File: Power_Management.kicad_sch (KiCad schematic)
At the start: 16 parts, among them J2 I2S_OR_LJ_OUT, Q1 MOSFET_SI2333DDS-T1-BE3, U4 SN74LVC1G07DBVR

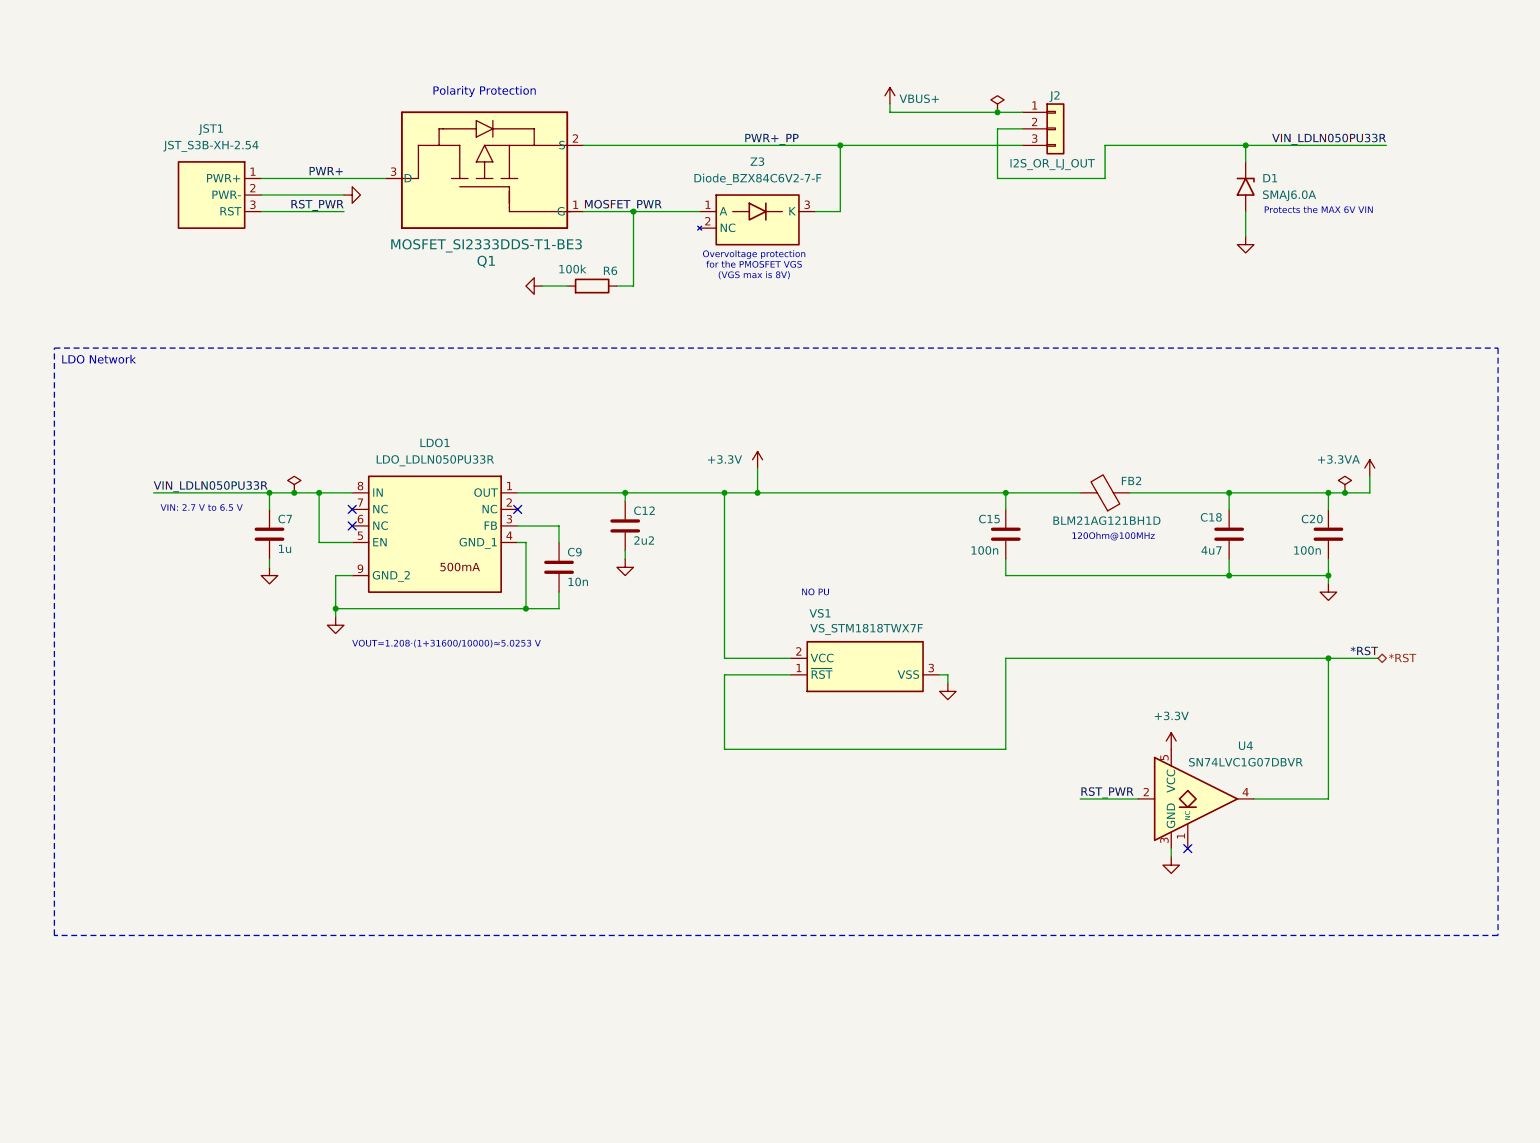
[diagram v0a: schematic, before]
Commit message: JLCPCB Check
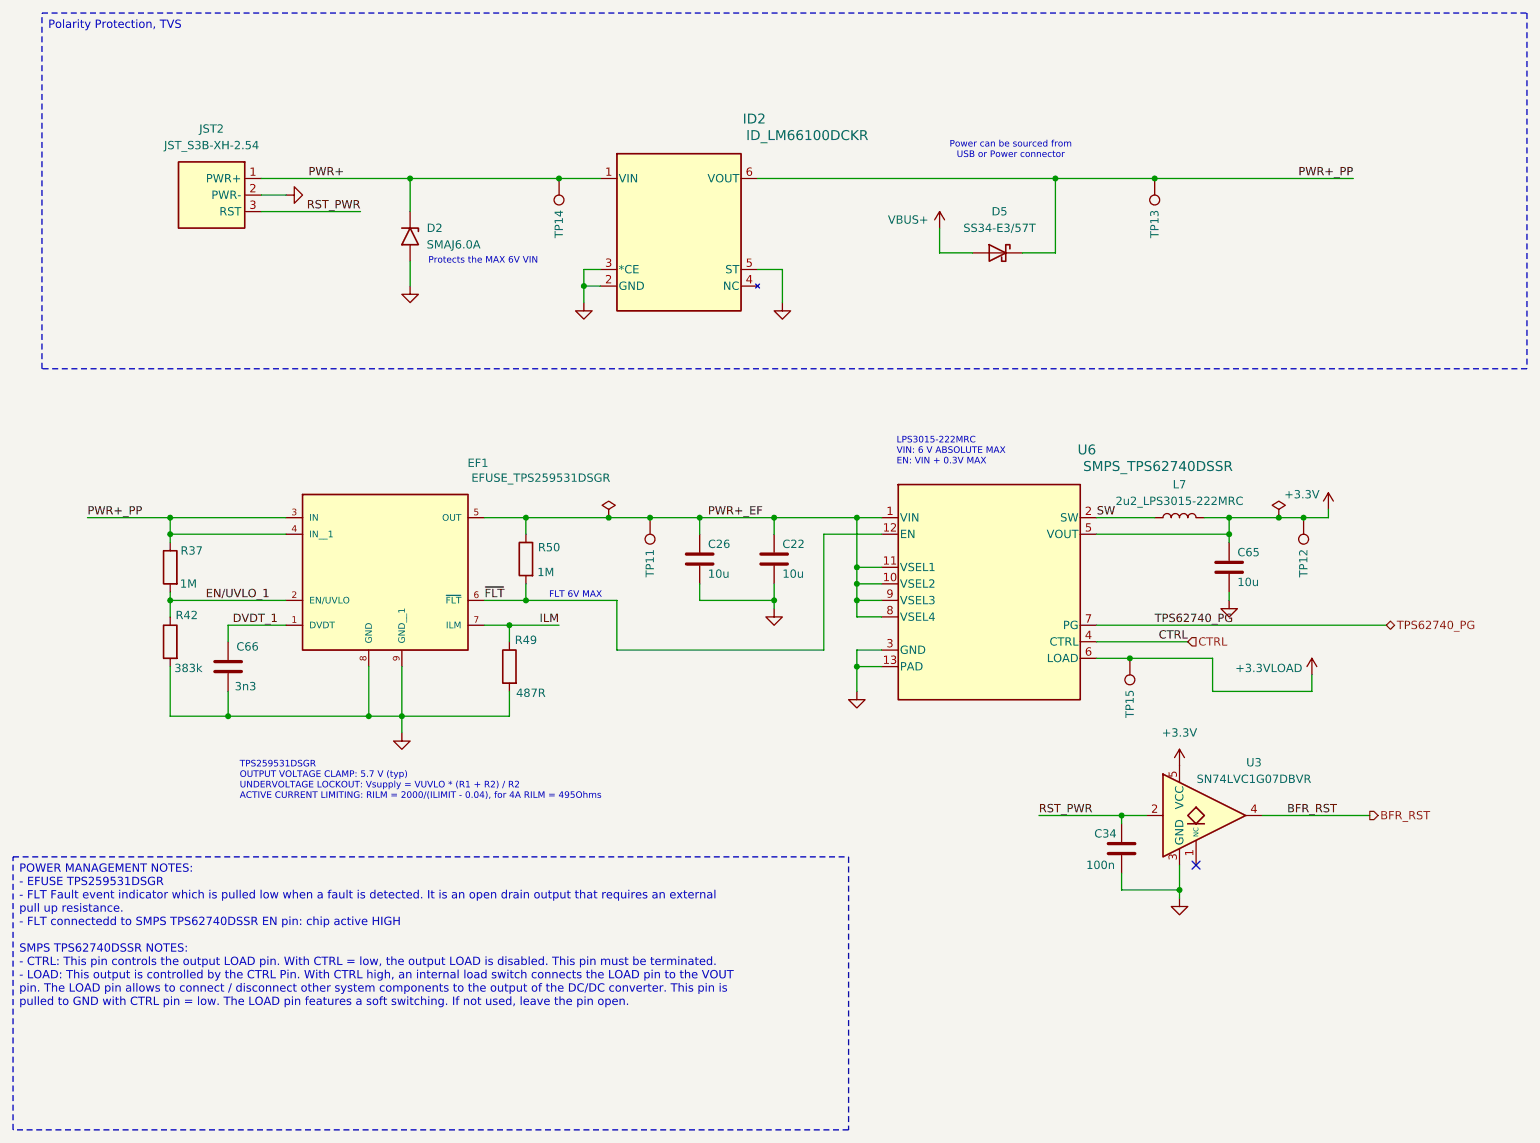
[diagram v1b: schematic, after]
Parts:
- removed C12: 2u2, Capacitor_SMD:C_0805_2012Metric, symbol Device:C
- removed C15, C20: 100n, Capacitor_SMD:C_0805_2012Metric, symbol Device:C
- removed C18: 4u7, Capacitor_SMD:C_0805_2012Metric, symbol Device:C
- removed C7: 1u, Capacitor_SMD:C_0805_2012Metric, symbol Device:C
- removed C9: 10n, Capacitor_SMD:C_0805_2012Metric, symbol Device:C
- removed D1: SMAJ6.0A, Personal_Project:DO-214AC-2, symbol Personal_Projects:DIODE_SMAJ6.0A
- removed FB2: BLM21AG121BH1D, Capacitor_SMD:C_0805_2012Metric, symbol Device:FerriteBead
- removed J2: I2S_OR_LJ_OUT, Connector_PinHeader_2.54mm:PinHeader_1x03_P2.54mm_Vertical, symbol Connector_Generic:Conn_01x03
- removed JST1: JST_S3B-XH-2.54, Personal_Project:JST_S3B-XH-SHDRRA3W64P0X250_1X3_990X1150X610P, symbol Personal_Projects:JST_S3B-XH-A-1_LF_SN
- removed LDO1: LDO_LDLN050PU33R, Package_DFN_QFN:DFN-8-1EP_3x3mm_P0.65mm_EP1.7x2.05mm, symbol Personal_Projects:LDO_LDLN050PUR
- removed Q1: MOSFET_SI2333DDS-T1-BE3, Personal_Project:MOSFET_ SI2333DDS_SOT_DS-T1-BE3_VIS, symbol Personal_Projects:MOSFET_SI2333DDS-T1-BE3
- removed R6: 100k, Resistor_SMD:R_0805_2012Metric, symbol Device:R
- removed U4: SN74LVC1G07DBVR, Package_TO_SOT_SMD:SOT-23-5, symbol 74xGxx:74LVC1G07
- removed VS1: VS_STM1818TWX7F, Personal_Project:SOT-23-3_SOT103P237X112-3N, symbol Personal_Projects:VS_STM1813LWX7F
- removed Z3: Diode_BZX84C6V2-7-F, Personal_Project:Diode_BZX84C6V2_SOT96P240X110-3N, symbol Personal_Projects:Diode_BZX84C6V2-7-F
- added C22, C26, C65: 10u, Capacitor_SMD:C_0603_1608Metric, symbol Device:C
- added C34: 100n, Capacitor_SMD:C_0805_2012Metric, symbol Device:C
- added C66: 3n3, Capacitor_SMD:C_0603_1608Metric, symbol Device:C
- added D2: SMAJ6.0A, Personal_Project:DO-214AC-2, symbol Personal_Projects:DIODE_SMAJ6.0A
- added D5: SS34-E3/57T, Diode_SMD:D_SMA, symbol Diode:SS34
- added EF1: EFUSE_TPS259531DSGR, Personal_Projects:EF_TPS259531DSGR, symbol Personal_Components:EFUSE_TPS259531DSGR
- added ID2: ID_LM66100DCKR, Personal_Projects:ID_LM66100DCKR, symbol Personal_Components:ID_LM66100DCKR
- added JST2: JST_S3B-XH-2.54, Personal_Project:JST_S3B-XH-SHDRRA3W64P0X250_1X3_990X1150X610P, symbol Personal_Projects:JST_S3B-XH-A-1_LF_SN
- added L7: 2u2_LPS3015-222MRC, Inductor_SMD:L_Coilcraft_LPS3010, symbol Device:L
- added R37, R50: 1M, Resistor_SMD:R_0603_1608Metric, symbol Device:R
- added R42: 383k, Resistor_SMD:R_0603_1608Metric, symbol Device:R
- added R49: 487R, Resistor_SMD:R_0603_1608Metric, symbol Device:R
- added TP11, TP12, TP13, TP14, TP15: TestPoint, TestPoint:TestPoint_Pad_1.5x1.5mm, symbol Connector:TestPoint
- added U3: SN74LVC1G07DBVR, Package_TO_SOT_SMD:SOT-23-5, symbol 74xGxx:74LVC1G07
- added U6: SMPS_TPS62740DSSR, Personal_Projects:SMPS_TPS62740DSSR, symbol Personal_Components:SMPS_TPS62740DSSR
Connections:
- net +3.3V: now also C65.1, L7.2, TP12.1, U3.5 (VCC), U6.5 (VOUT)
- net GND: now also C22.2, C26.2, C34.2, C65.2, C66.1, D2.2 (A), EF1.8 (GND), EF1.9 (GND__1), ID2.2 (GND), ID2.3 (*CE), ID2.5 (ST), JST2.2 (PWR-), R42.2, R49.2, U3.3 (GND), U6.13 (PAD), U6.3 (GND)
- net PWR+: now also D2.1 (K), ID2.1 (VIN), JST2.1 (PWR+), TP14.1
- net PWR+_PP: now also D5.1 (K), EF1.3 (IN), EF1.4 (IN__1), ID2.6 (VOUT), R37.1, TP13.1
- net RST_PWR: now also C34.1, JST2.3 (RST), U3.2
- net VBUS+: now also D5.2 (A)
- new net +3.3VLOAD: TP15.1, U6.6 (LOAD)
- new net BFR_RST: U3.4
- new net CTRL: U6.4 (CTRL)
- new net DVDT_1: C66.2, EF1.1 (DVDT)
- new net EN/UVLO_1: EF1.2 (EN/UVLO), R37.2, R42.1
- new net ILM: EF1.7 (ILM), R49.1
- new net PWR+_EF: C22.1, C26.1, EF1.5 (OUT), R50.1, TP11.1, U6.1 (VIN), U6.10 (VSEL2), U6.11 (VSEL1), U6.8 (VSEL4), U6.9 (VSEL3)
- new net SW: L7.1, U6.2 (SW)
- new net TPS62740_PG: U6.7 (PG)
- new net ~{FLT}: EF1.6 (~{FLT}), R50.2, U6.12 (EN)
- no-connect marks 4 -> 1
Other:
- note added: "FLT 6V MAX"
- note added: "LPS3015-222MRC VIN: 6 V ABSOLUTE MAX EN: VIN + 0.3V MAX"
- note added: "Power can be sourced from USB or Power connector"
- note added: "TPS259531DSGR OUTPUT VOLTAGE CLAMP: 5.7 V (typ) UNDERVOLTAGE LOCKOUT: Vsupply = VUVLO * (R1 + R2) / R2 ACTIVE CURRENT LIMITING: RILM = 2000/(ILIMIT - 0.04), for 4A RILM = 495Ohms"
- note removed: "120Ohm@100MHz"
- note removed: "NO PU"
- note removed: "Overvoltage protection for the PMOSFET VGS (VGS max is 8V)"
- note removed: "Polarity Protection"
- note removed: "VIN: 2.7 V to 6.5 V"
- note removed: "VOUT​=1.208⋅(1+31600/10000)≈5.0253 V"
